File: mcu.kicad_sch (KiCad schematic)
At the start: 4 parts, among them U3 STM32F733VETx

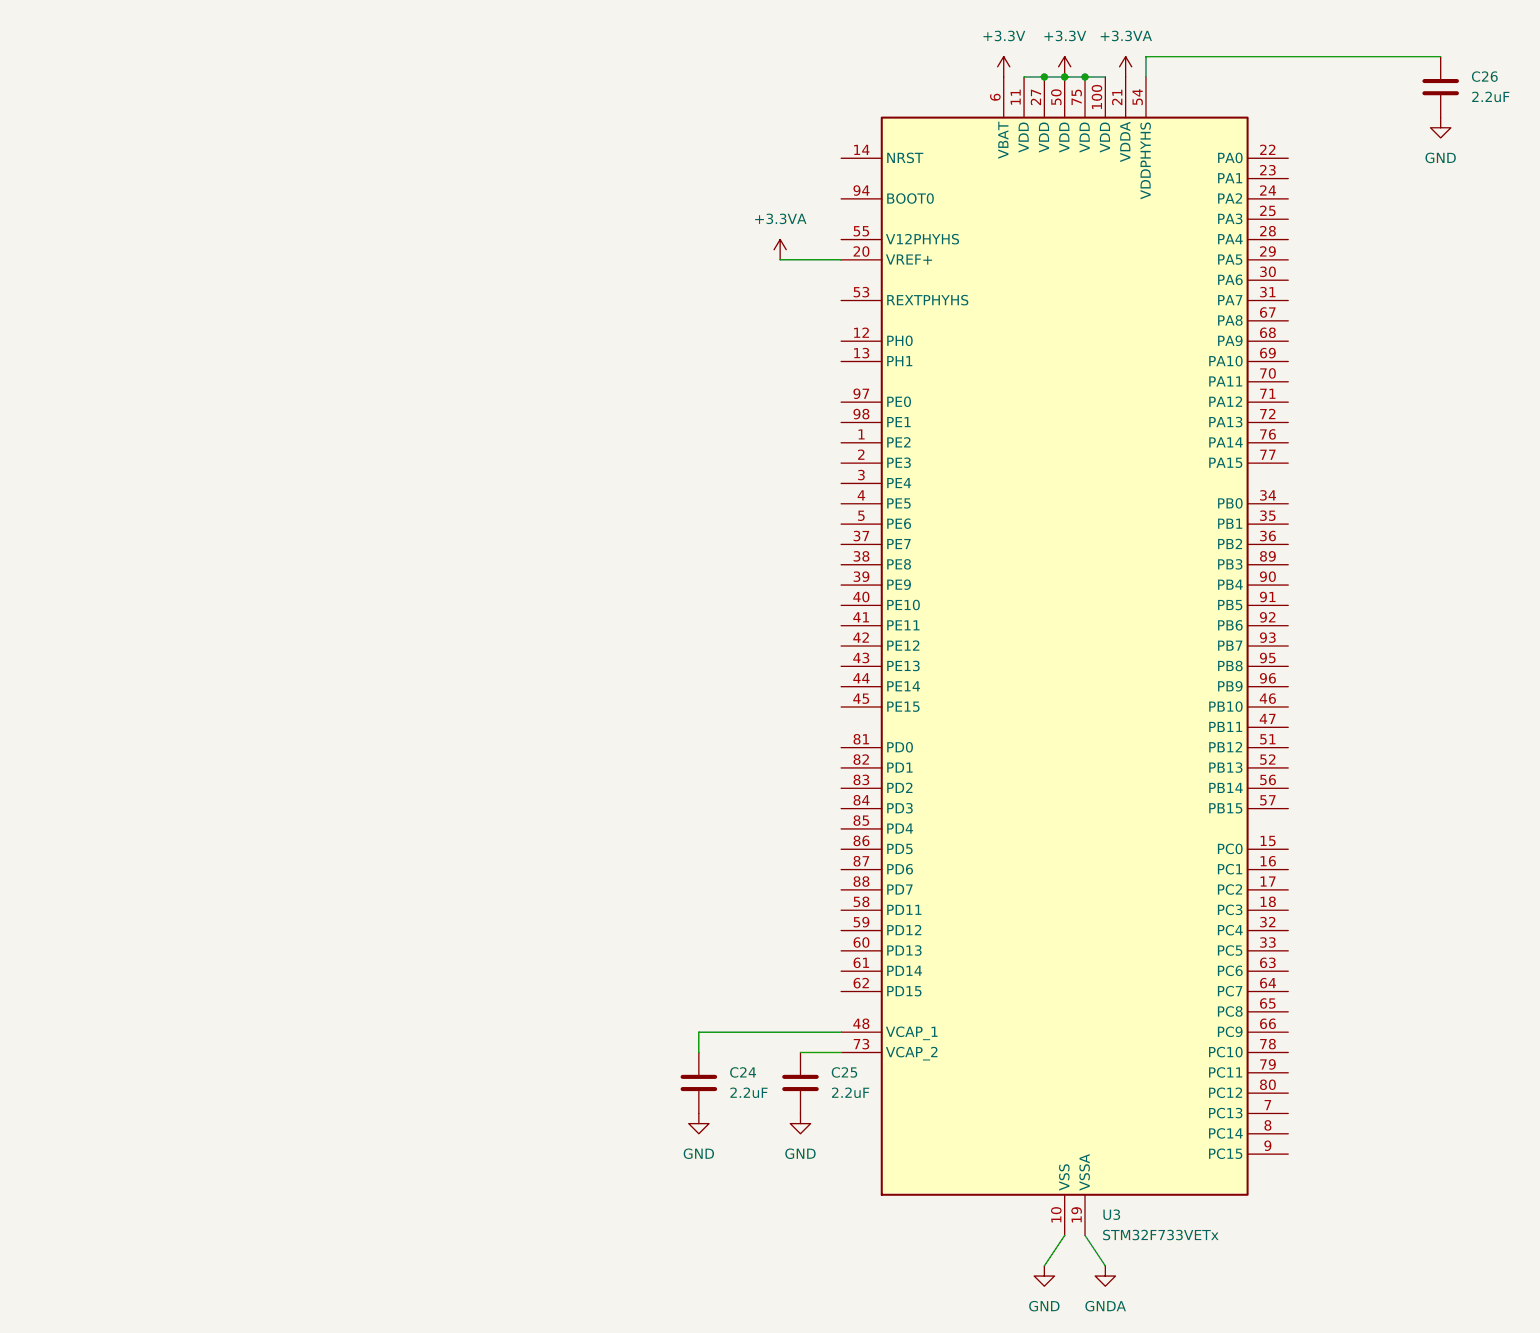
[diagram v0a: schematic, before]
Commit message: finish power caps
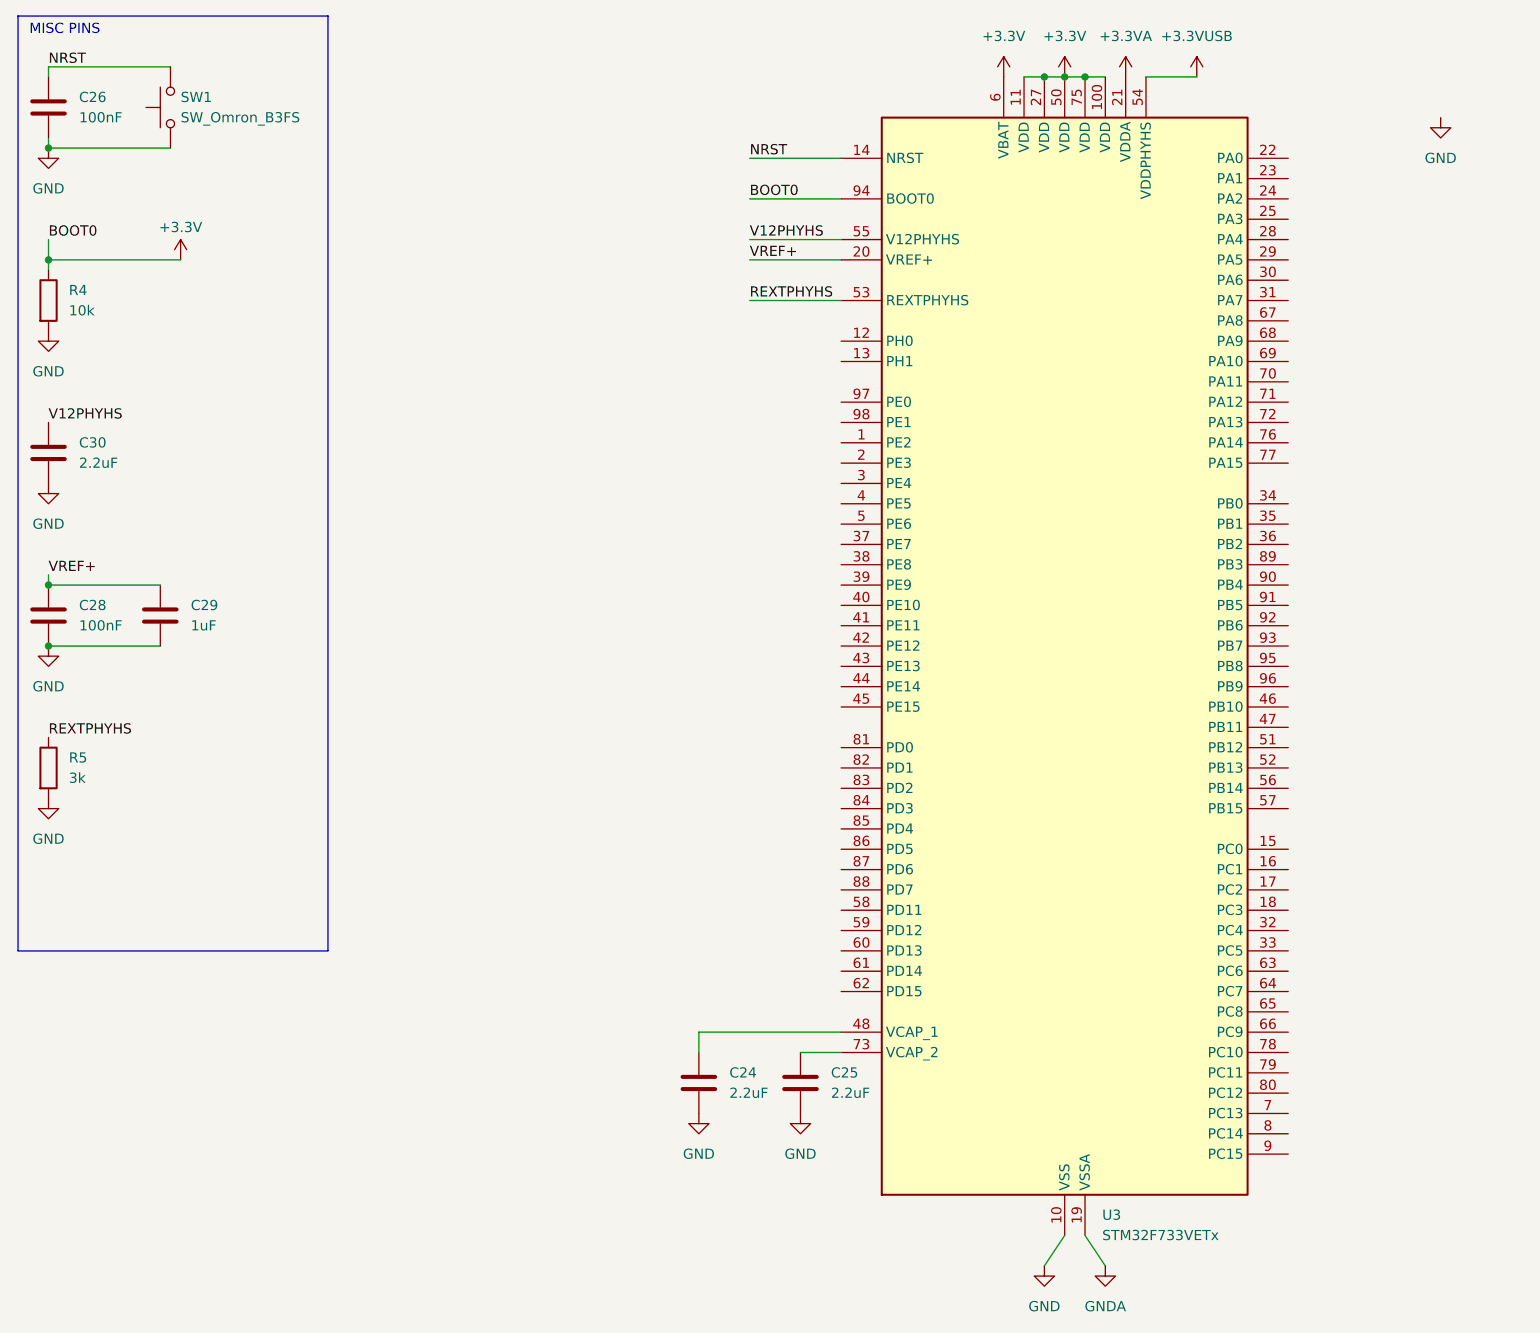
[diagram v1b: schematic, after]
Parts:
- added C28: 100nF, symbol Device:C
- added C29: 1uF, symbol Device:C
- added C30: 2.2uF, symbol Device:C
- added R4: 10k, symbol Device:R
- added R5: 3k, symbol Device:R
- added SW1: SW_Omron_B3FS, symbol Switch:SW_Omron_B3FS
- C26: value 2.2uF -> 100nF
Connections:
- net +3.3V: now also U3.94 (BOOT0), R4.1
- net +3.3VA: no longer U3.20 (VREF+)
- net GND: now also C28.2, C29.2, C30.2, R4.2, R5.2, SW1.1
- net NRST: now reaches U3.14 (NRST)
- net NRST: now also C26.1, SW1.2
- net REXTPHYHS: now reaches U3.53 (REXTPHYHS)
- net REXTPHYHS: now also R5.1
- net +3.3VUSB: now reaches U3.54 (VDDPHYHS)
- net +3.3VUSB: no longer C26.1
- net V12PHYHS: now reaches U3.55 (V12PHYHS)
- net V12PHYHS: now also C30.1
- new net VREF+: C28.1, C29.1, U3.20 (VREF+)
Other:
- note added: "MISC PINS"
